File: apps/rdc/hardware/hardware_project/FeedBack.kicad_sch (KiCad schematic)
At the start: 40 parts, among them Q10 DTC143ZCAT116, Q11 DTC143ZCAT116, U2 TLV2171IDR, U3 TLV431BFTA, U4 TLV431BFTA, U5 CD4053BPWRG3, U6 CD4053BPWRG3

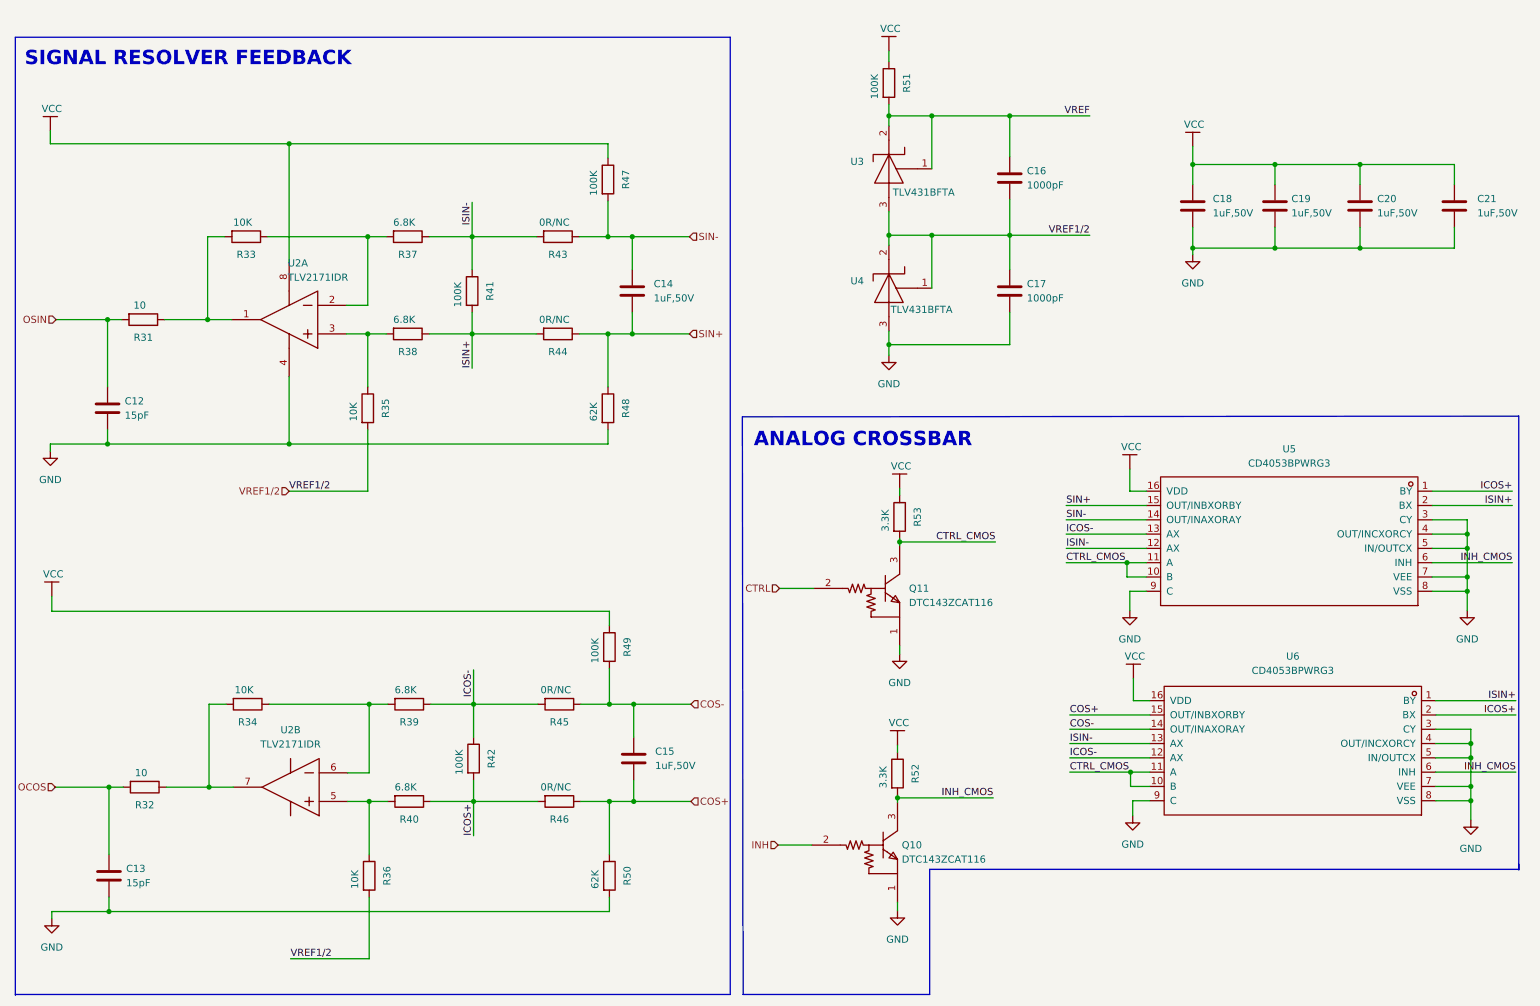
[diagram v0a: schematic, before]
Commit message: hpm apps release v1.8.0
Signed-off-by: zhangeg <engui.zhang@hpmicro.com>
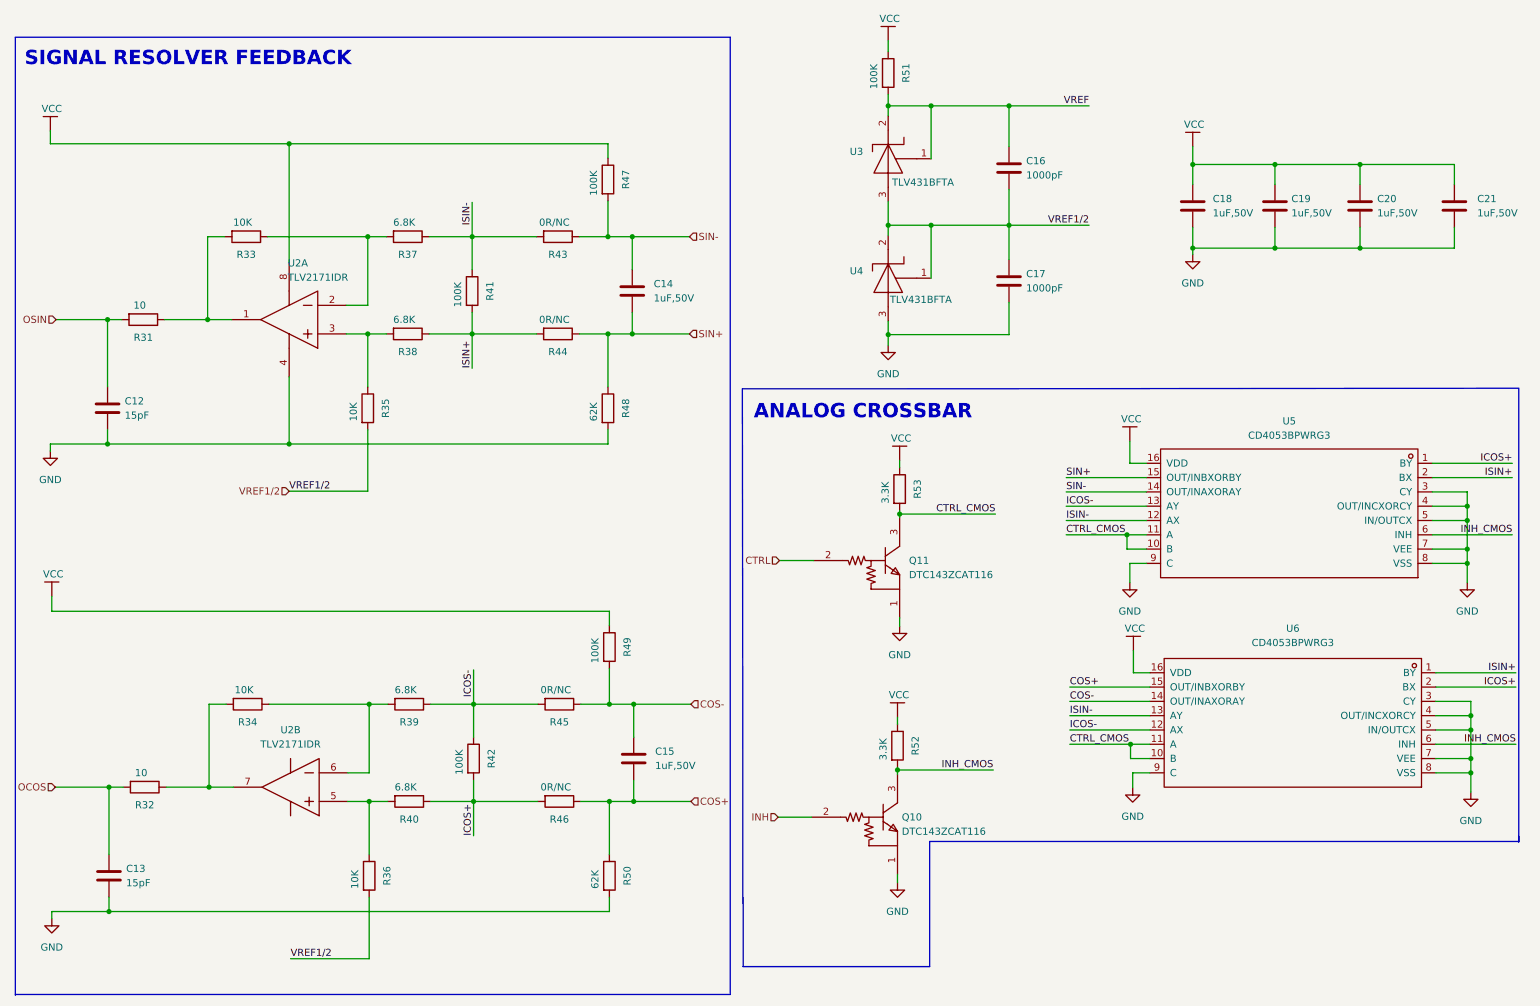
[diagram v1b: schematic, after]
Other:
- moved on the sheet: C16, C17, Q10, Q11, R51, R52, R53, U3, U4, U5, U6
